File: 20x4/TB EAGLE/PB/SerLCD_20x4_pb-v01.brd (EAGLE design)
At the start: 73.7 x 139.7 mm, 21 parts, among them J1 AVR_PROG, J3 SER_LCD16X2, U1 5V Flying Jalapeno, U2 74LVC4066_MUX_1:1_X4

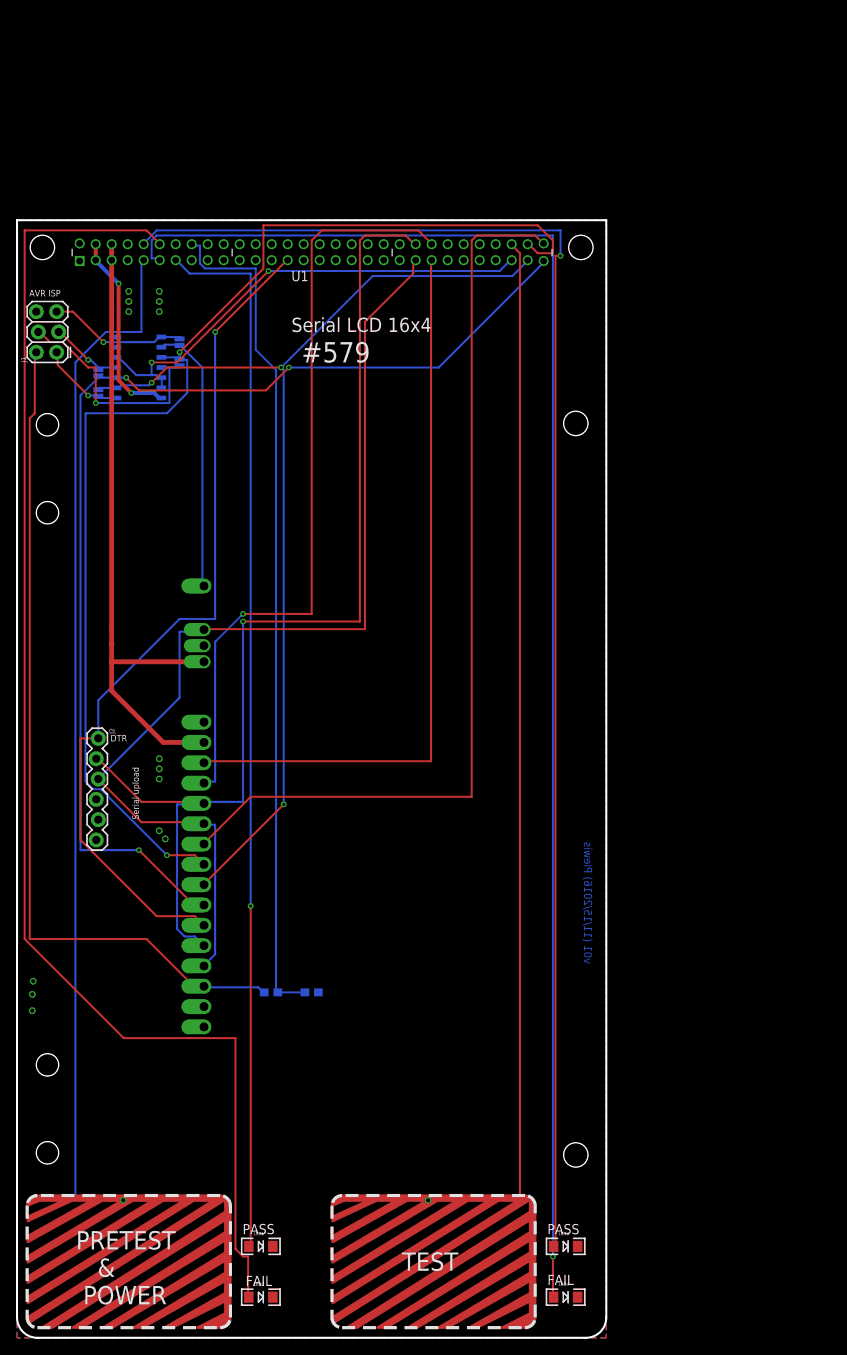
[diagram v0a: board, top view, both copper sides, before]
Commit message: finshed up 20x4, RFR
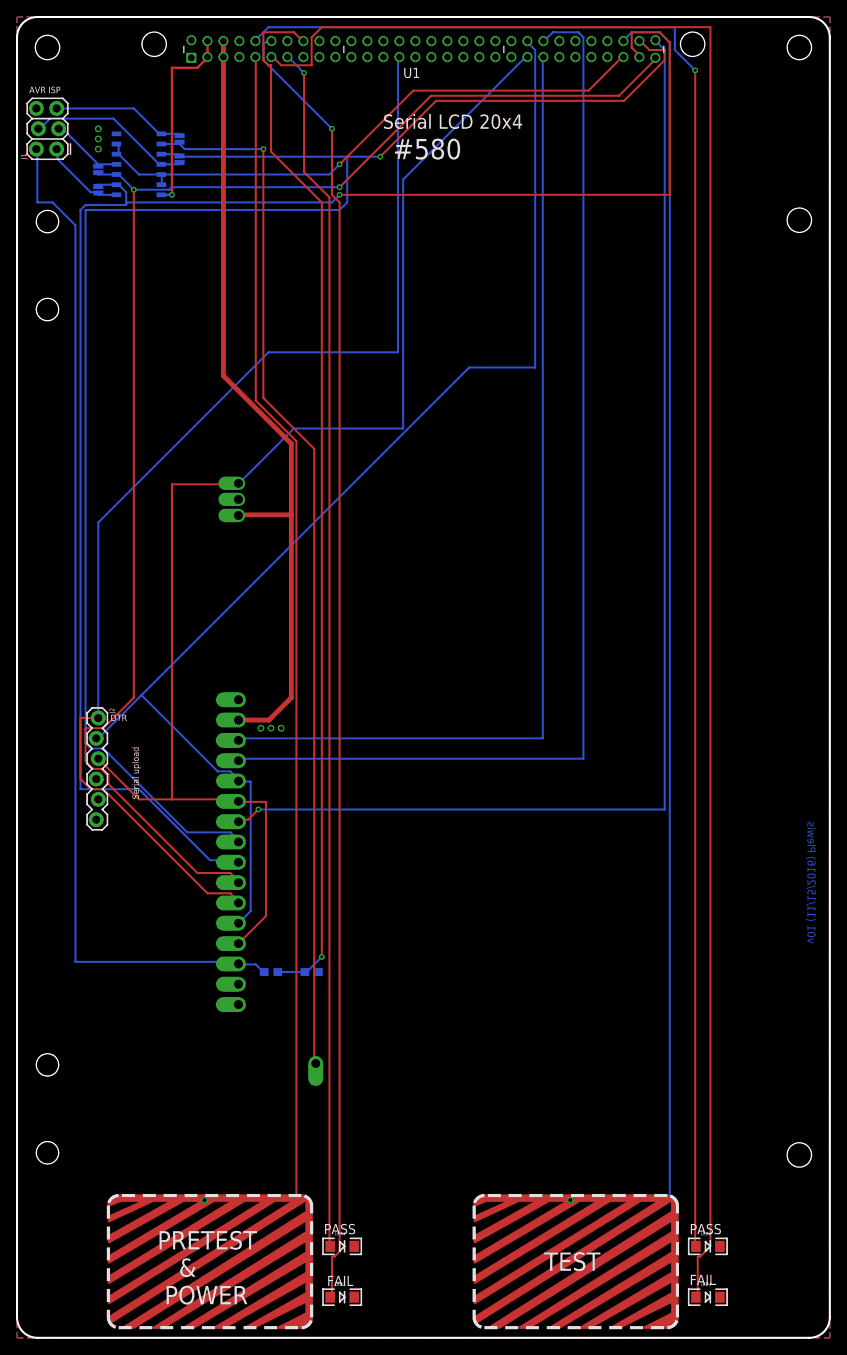
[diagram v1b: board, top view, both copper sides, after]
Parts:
- added U$1, U$2: (no value), SparkFun:STAND-OFF-TIGHT
- J3: value SER_LCD16X2 -> SER_LCD20X4; device SerLCD_dimensions:SER_LCD_16X2 -> SerLCD_dimensions:SER_LCD_20X4
- moved U$3 37.8 mm to (97.8, 139.7)
- moved U1 29.0 mm to (50.8, 165.1)
- moved J3 28.1 mm to (85.1, 31.8)
- moved U$8 27.9 mm to (97.8, 22.9)
- moved JP3 25.4 mm to (20.3, 149.9)
- moved J1 25.4 mm to (5.08, 148.6)
- moved JP2 25.4 mm to (10.2, 146.1)
- moved U2 25.4 mm to (15.2, 146.1)
- moved JP1 25.4 mm to (10.2, 143.5)
- moved JP4 25.4 mm to (20.3, 147.3)
- moved U$6 25.4 mm to (0.00, 124.5)
- moved LED3 17.8 mm to (86.4, 11.4)
- moved LED4 17.8 mm to (86.4, 5.08)
- moved 2 17.8 mm to (69.8, 10.2)
- moved LED1 10.2 mm to (40.6, 11.4)
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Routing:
- net RST: track 34.0 -> 130.4 mm, vias 0 -> 1
- net MISO: track 129.4 -> 203.9 mm, vias 3 -> 1
- net MOSI: track 149.6 -> 202.9 mm, vias 2 -> 1
- net SCL: track 95.4 -> 139.1 mm, vias 1 -> 0
- net SCK: track 141.6 -> 179.0 mm, vias 3 -> 2
- net DTR_FJ: track 107.0 -> 143.8 mm, vias 1 -> 0
- net TX1_FJ: track 130.0 -> 166.5 mm
- net CS: track 115.1 -> 150.5 mm, vias 0 -> 1
- net N$2: track 131.4 -> 163.9 mm
- net N$6: track 186.6 -> 219.1 mm, vias 1 -> 0
- net SDA: track 91.1 -> 123.3 mm
- net N$1: track 129.6 -> 156.5 mm
- net N$5: track 180.7 -> 206.7 mm
- net N$7: track 105.7 -> 130.5 mm, vias 0 -> 1
- net 3.3_VCC: track 105.9 -> 129.0 mm
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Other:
- board size 73.7 x 139.7 mm -> 101.6 x 165.1 mm
- board text added: "#580"
- board text added: "Serial LCD 20x4"
- board text removed: "#579"
- board text removed: "Serial LCD 16x4"
